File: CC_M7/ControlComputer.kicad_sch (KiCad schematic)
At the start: 39 parts, among them J1 1x03_BootPin, U1 STM32H743VITx, Y1 32MHz

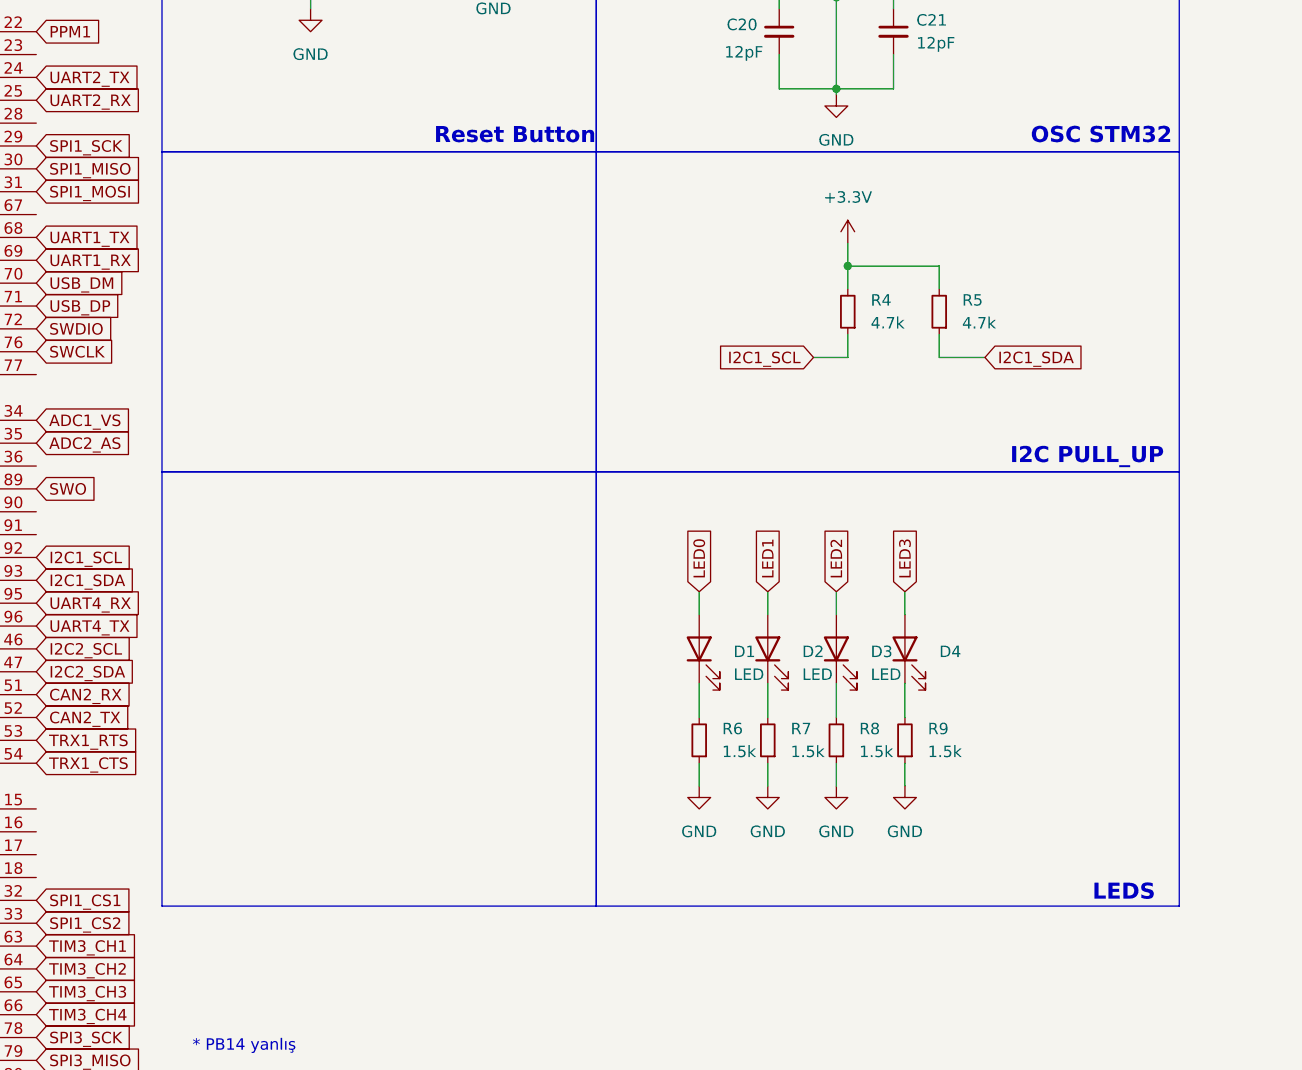
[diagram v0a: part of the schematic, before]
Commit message: nrf
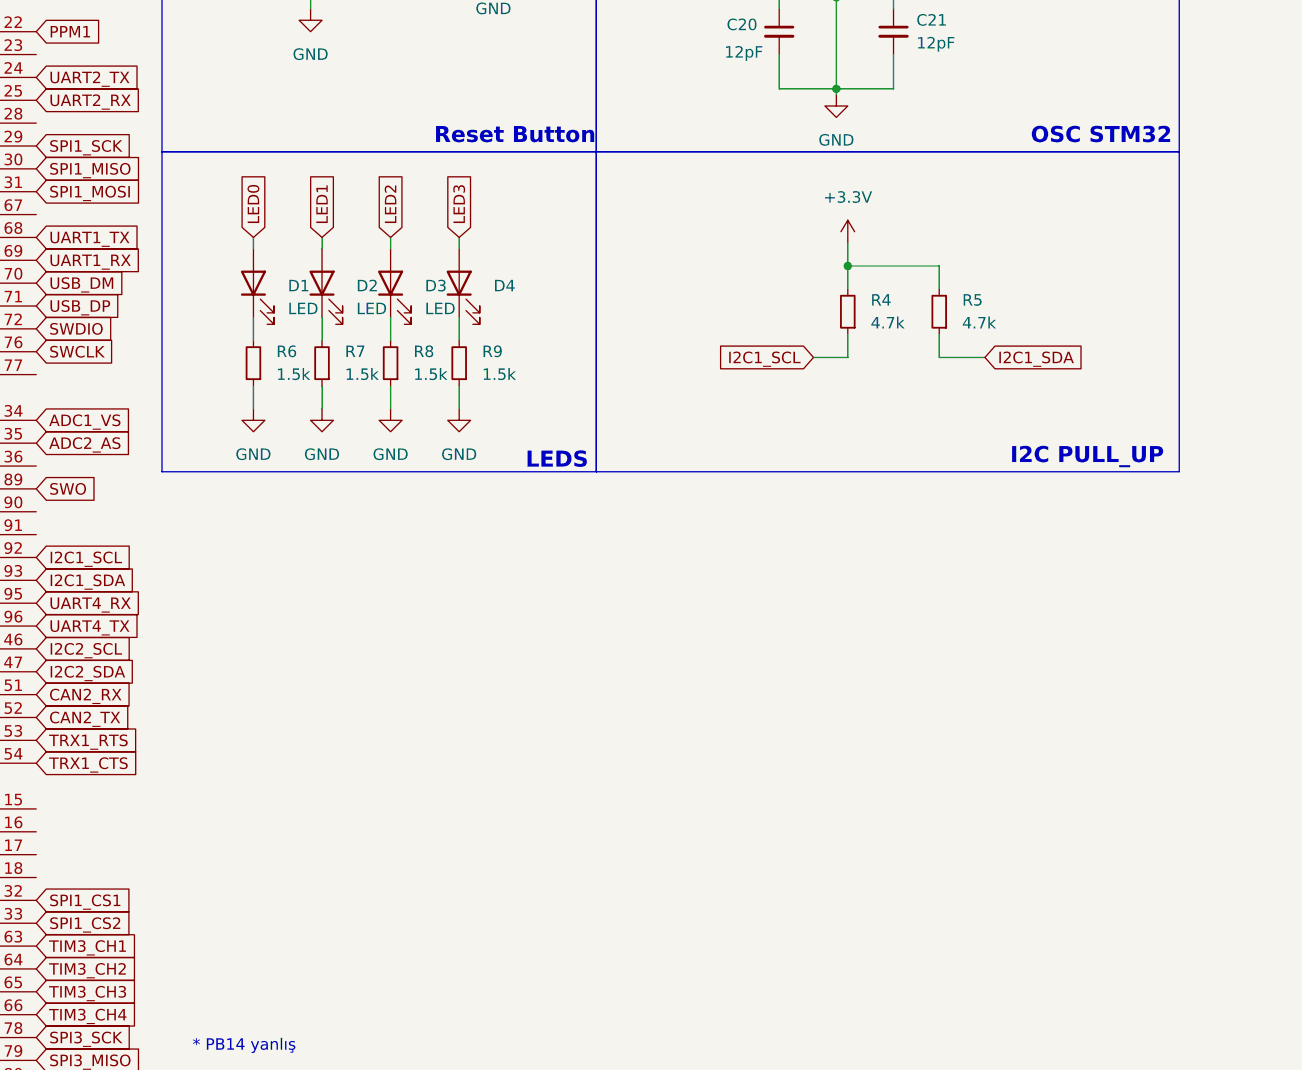
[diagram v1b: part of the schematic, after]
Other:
- moved on the sheet: D1, D2, D3, D4, R6, R7, R8, R9

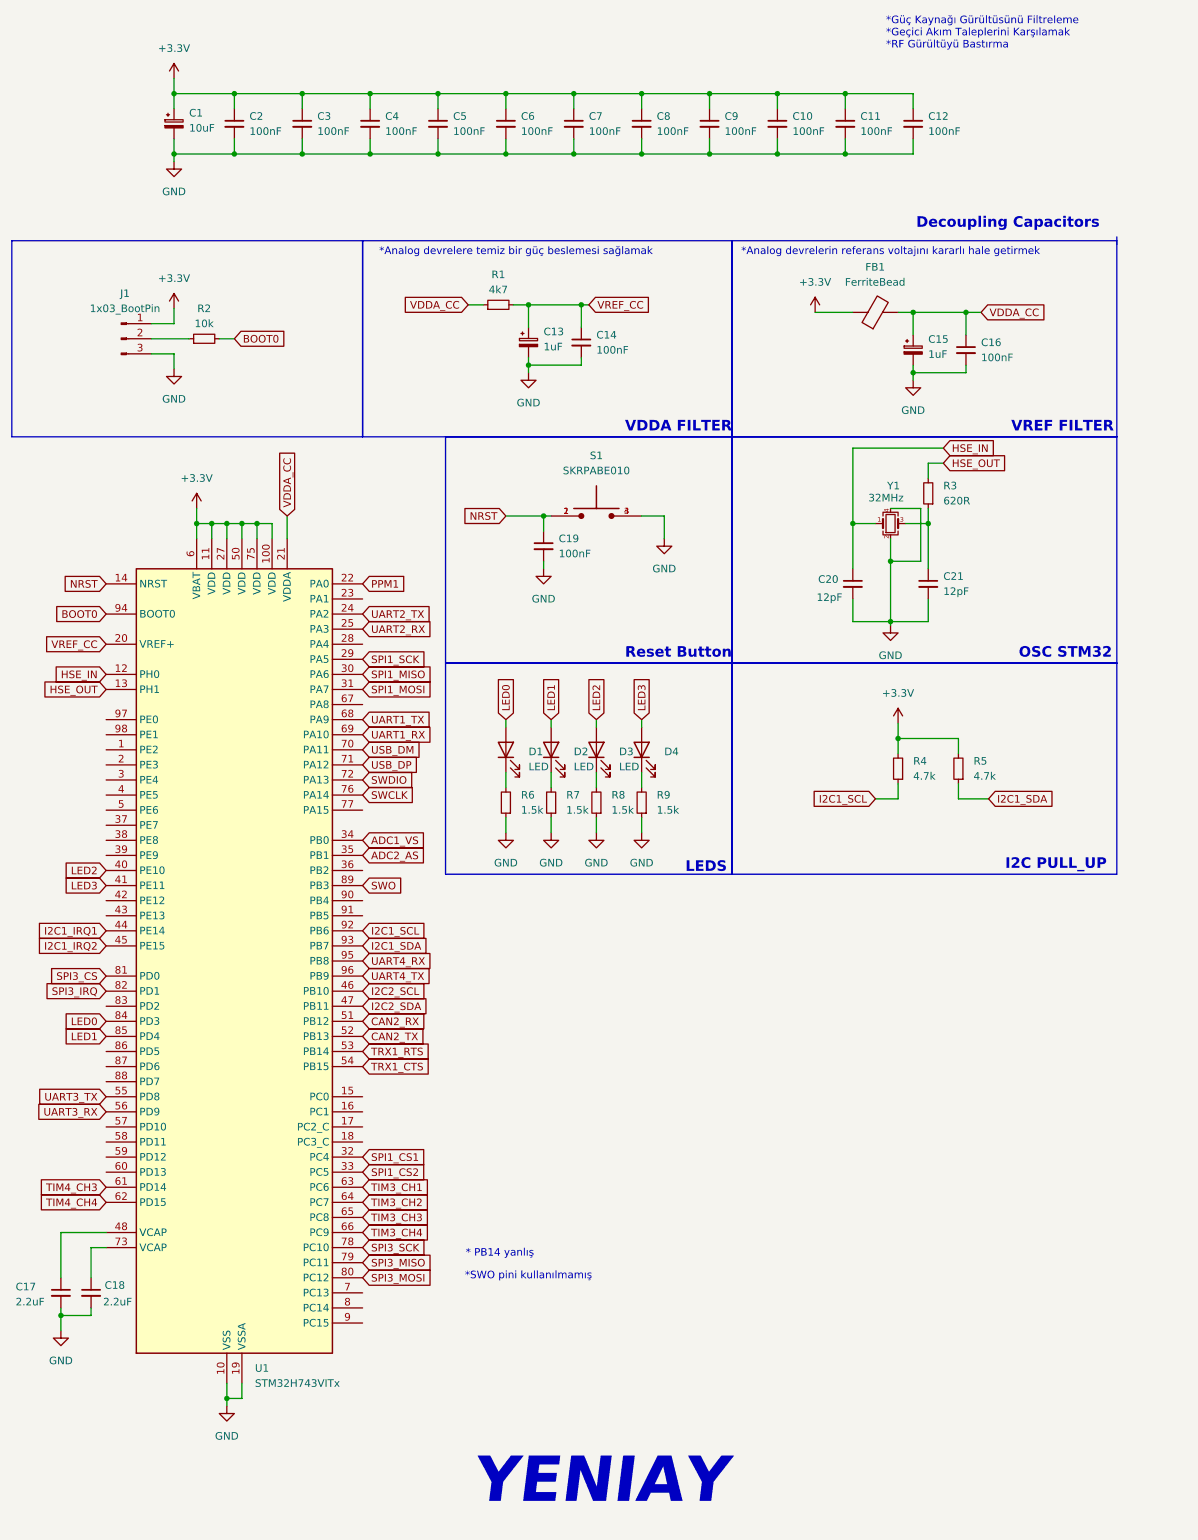
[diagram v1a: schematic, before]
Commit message: final schematic 6 warning
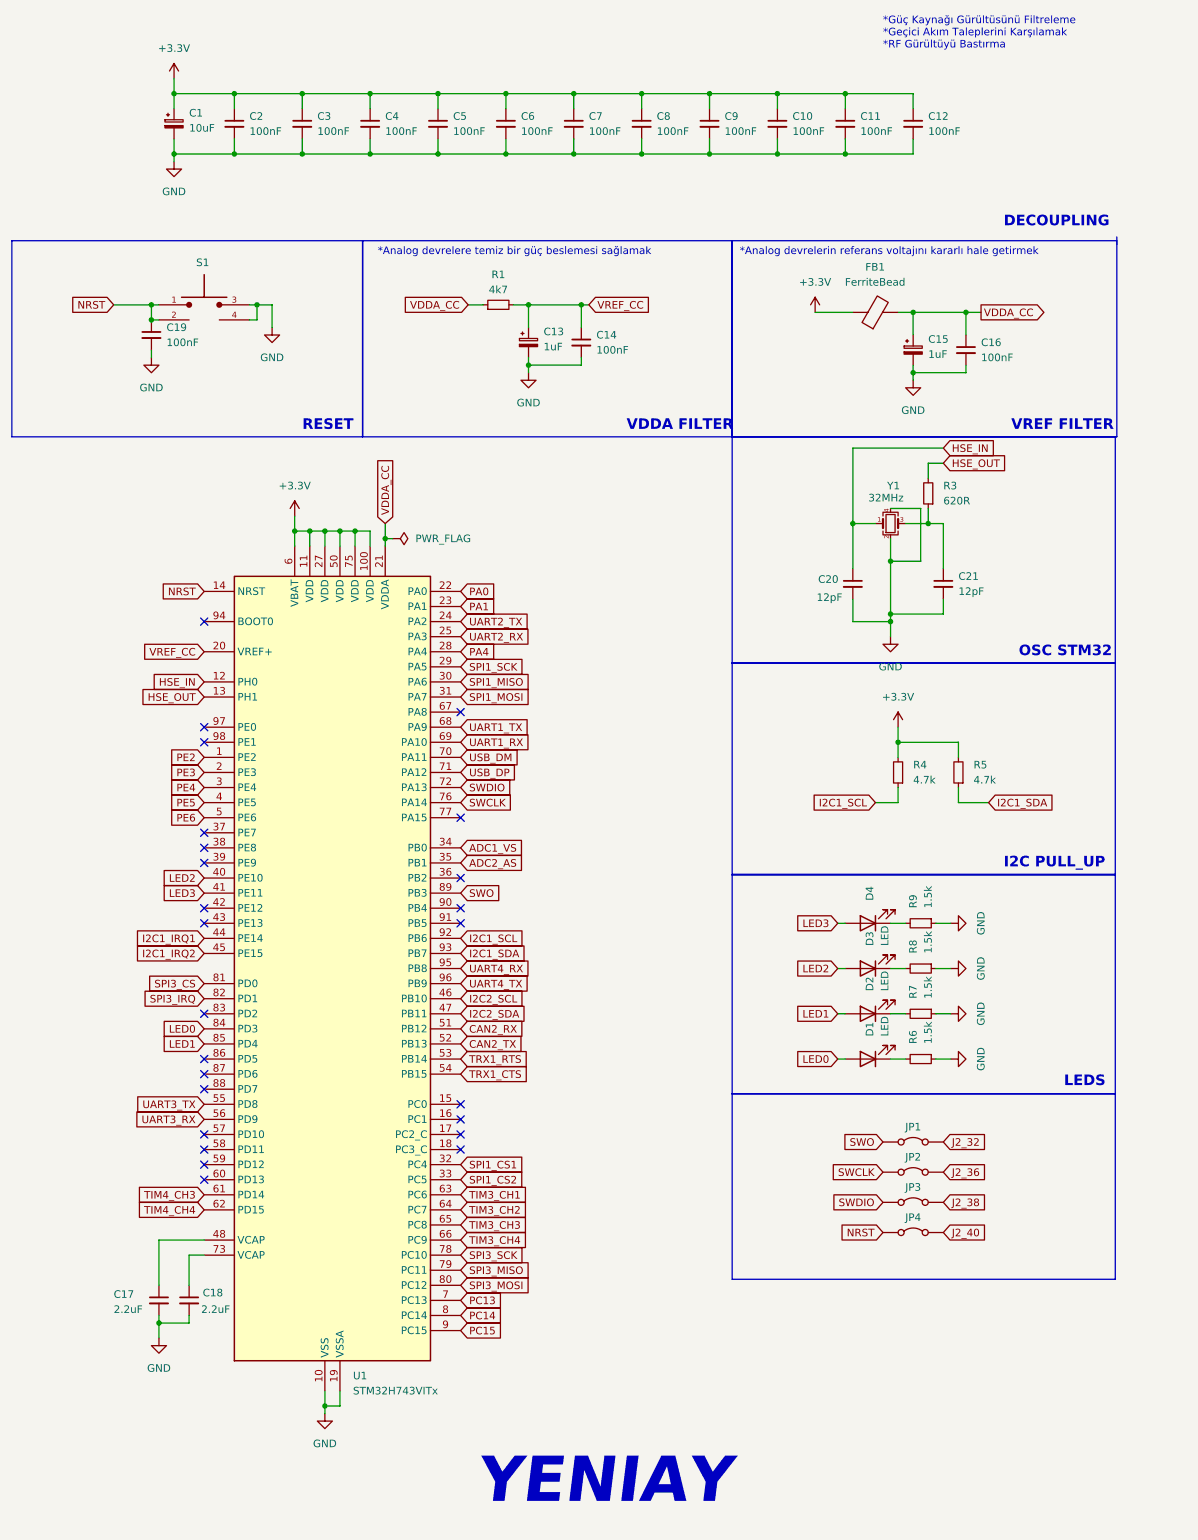
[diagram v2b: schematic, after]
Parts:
- removed J1: 1x03_BootPin, symbol Connector:Conn_01x03_Pin
- removed R2: 10k, symbol Device:R_Small
- added JP1, JP2, JP3, JP4: SWDIO, symbol Jumper:Jumper_2_Bridged
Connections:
- net I2C1_SDA  is gone; now on net I2C1_SDA: U1.93 (PB7)
- net NRST: now also JP4.1 (A)
- net SWCLK: now also JP2.1 (A)
- net SWDIO: now also JP3.1 (A)
- net SWO: now also JP1.1 (A)
- net PE2: now reaches U1.1 (PE2)
- net PE3: now reaches U1.2 (PE3)
- net PA1: now reaches U1.23 (PA1)
- net PA4: now reaches U1.28 (PA4)
- net PE4: now reaches U1.3 (PE4)
- net PE5: now reaches U1.4 (PE5)
- net PE6: now reaches U1.5 (PE6)
- net PC13: now reaches U1.7 (PC13)
- net PC14: now reaches U1.8 (PC14)
- net PC15: now reaches U1.9 (PC15)
- net BOOT0: no longer names the net of U1.94 (BOOT0)
- net PPM1 renamed PA0
- new net J2_32: JP1.2 (B)
- new net J2_36: JP2.2 (B)
- new net J2_38: JP3.2 (B)
- new net J2_40: JP4.2 (B)
- no-connect marks 0 -> 25
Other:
- note added: "DECOUPLING"
- note added: "RESET"
- note removed: "* PB14 yanlış"
- note removed: "*SWO pini kullanılmamış"
- note removed: "Decoupling Capacitors"
- note removed: "Reset Button"
- moved on the sheet: C17, C18, C19, C21, D1, D2, D3, D4, R4, R5, R6, R7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

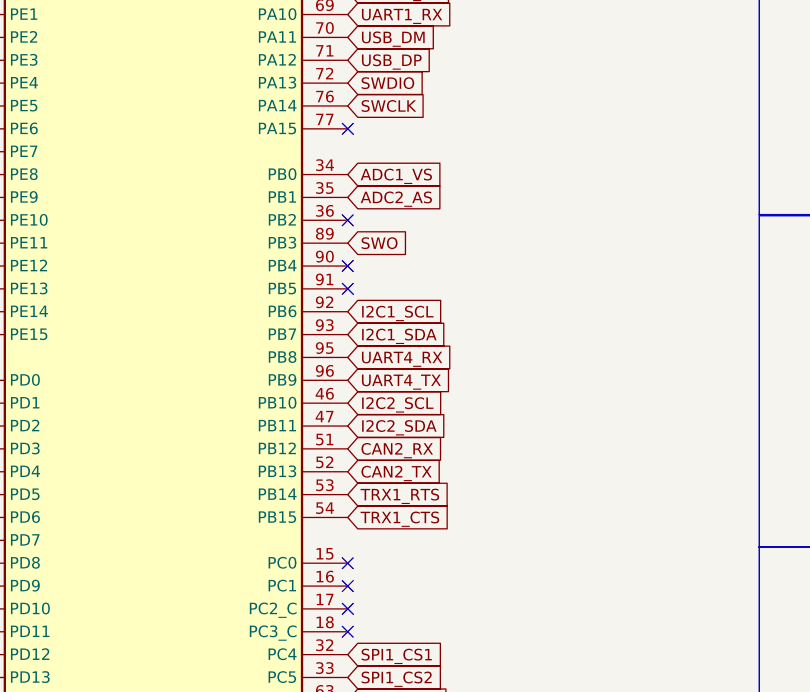
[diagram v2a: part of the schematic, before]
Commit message: Changes updated @ CCM7.docx
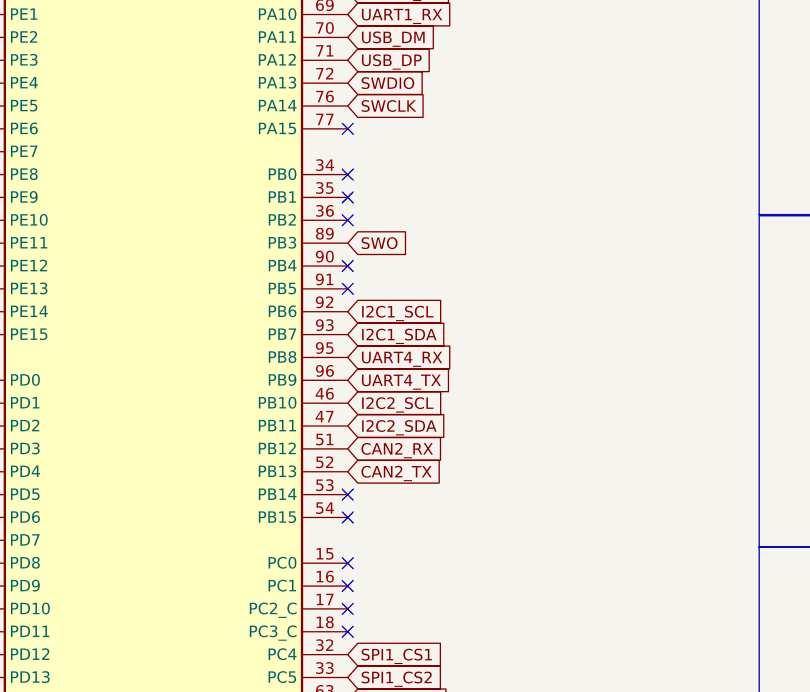
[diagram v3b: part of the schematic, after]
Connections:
- net ADC1_VS: no longer names the net of U1.34 (PB0)
- net ADC2_AS: no longer names the net of U1.35 (PB1)
- net TRX1_CTS: no longer names the net of U1.54 (PB15)
- net TRX1_RTS: no longer names the net of U1.53 (PB14)
- no-connect marks 25 -> 29
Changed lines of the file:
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@@
 	)
 	(no_connect
+		(at 87.63 190.5)
+	)
+	(no_connect
 		(at 87.63 205.74)
 	)
 	(no_connect
+		(at 87.63 193.04)
+	)
+	(no_connect
 		(at 87.63 203.2)
 	)
@@
 	)
 	(no_connect
+		(at 87.63 157.48)
+	)
+	(no_connect
 		(at 44.45 208.28)
 	)
@@
 	)
 	(no_connect
+		(at 87.63 154.94)
+	)
+	(no_connect
 		(at 44.45 134.62)
 	)
@@
 		)
 	)
-	(global_label "ADC1_VS"
-		(shape input)
-		(at 87.63 154.94 0)
-		(fields_autoplaced yes)
-		(effects
-			(font
-				(size 1.27 1.27)
-			)
-			(justify left)
-		)
-		(property "Intersheetrefs" "${INTERSHEET_REFS}"
-			(at 98.719 154.94 0)
-			(effects
-				(font
-					(size 1.27 1.27)
-				)
-				(justify left)
-				(hide yes)
-			)
-		)
-	)
 	(global_label "TIM4_CH3"
 		(shape input)
@@
 		)
 	)
-	(global_label "ADC2_AS"
-		(shape input)
-		(at 87.63 157.48 0)
-		(fields_autoplaced yes)
-		(effects
-			(font
-				(size 1.27 1.27)
-			)
-			(justify left)
-		)
-		(property "Intersheetrefs" "${INTERSHEET_REFS}"
-			(at 98.719 157.48 0)
-			(effects
-				(font
-					(size 1.27 1.27)
-				)
-				(justify left)
-				(hide yes)
-			)
-		)
-	)
 	(global_label "SPI1_MOSI"
 		(shape input)
@@
 		)
 	)
-	(global_label "TRX1_CTS"
-		(shape input)
-		(at 87.63 193.04 0)
-		(fields_autoplaced yes)
-		(effects
-			(font
-				(size 1.27 1.27)
-			)
-			(justify left)
-		)
-		(property "Intersheetrefs" "${INTERSHEET_REFS}"
-			(at 99.6865 193.04 0)
-			(effects
-				(font
-					(size 1.27 1.27)
-				)
-				(justify left)
-				(hide yes)
-			)
-		)
-	)
 	(global_label "SPI3_SCK"
 		(shape input)
@@
 			(effects
 				(font
-					(size 1.27 1.27)
-				)
-				(justify left)
-				(hide yes)
-			)
-		)
-	)
-	(global_label "TRX1_RTS"
-		(shape input)
-		(at 87.63 190.5 0)
-		(fields_autoplaced yes)
-		(effects
-			(font
-				(size 1.27 1.27)
-			)
-			(justify left)
-		)
-		(property "Intersheetrefs" "${INTERSHEET_REFS}"
-			(at 99.6865 190.5 0)
-			(effects
-				(font
